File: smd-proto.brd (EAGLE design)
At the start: 79.2 x 43.9 mm, 65 parts

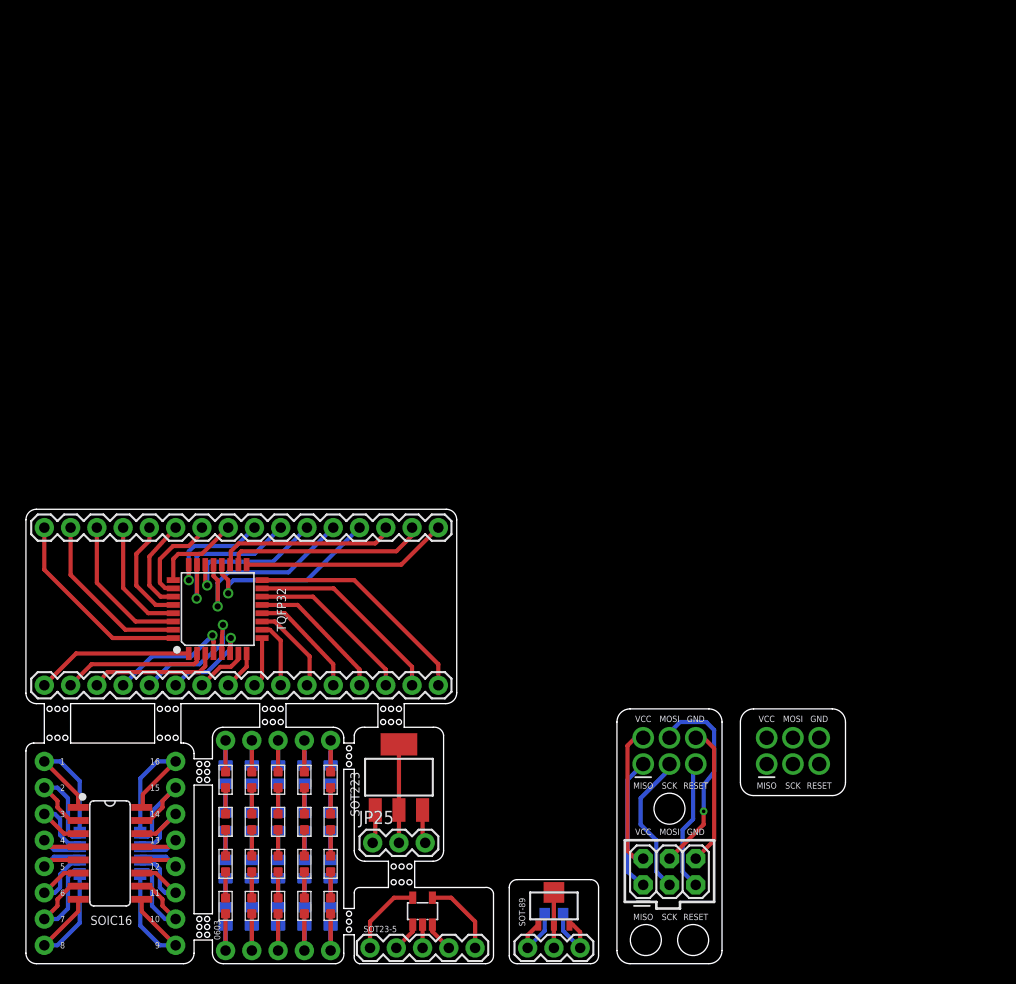
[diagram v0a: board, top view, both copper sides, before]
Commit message: Added bunch of boards and outline
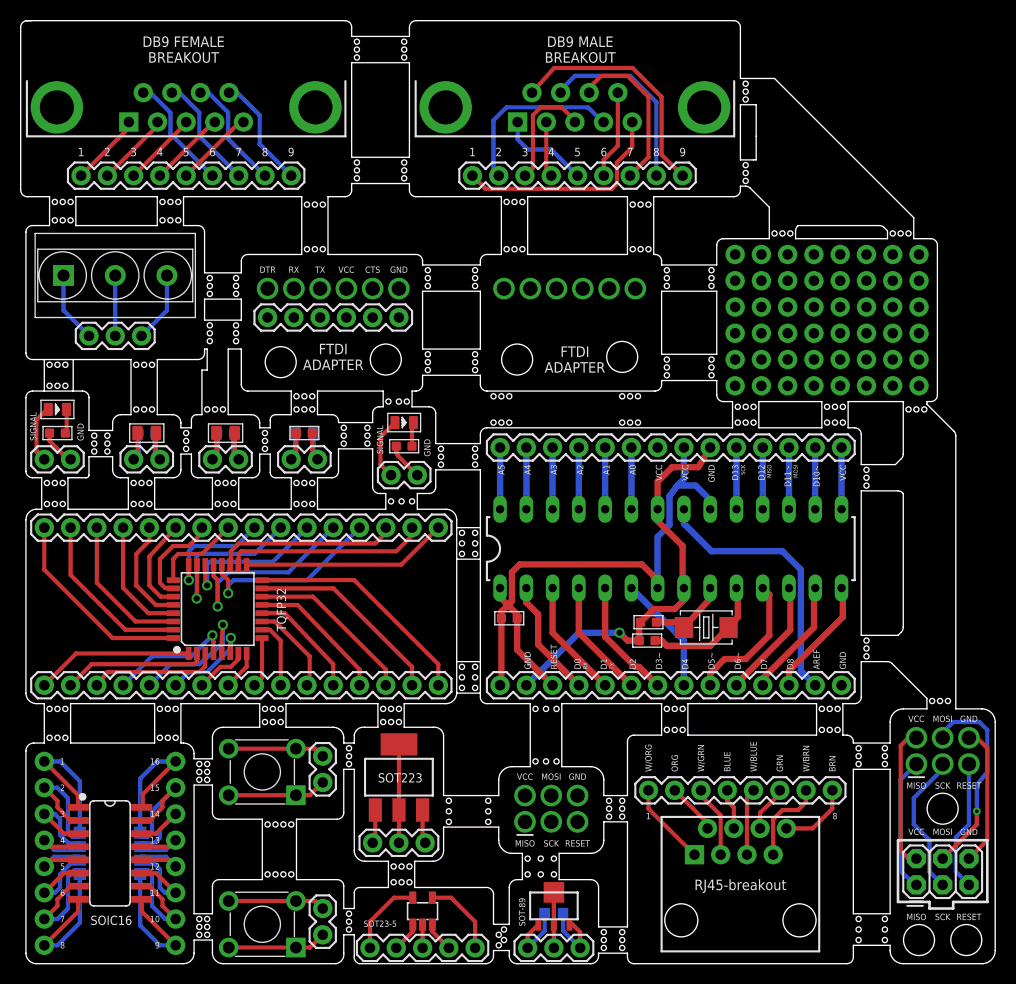
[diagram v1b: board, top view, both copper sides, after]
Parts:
- removed C10, C11, C12, C13, C14, C15, C16, C17, C18, C19, C20, C21, C3, C4, C5, C6, C7, C8, C9: 0.5PF 50V, Seeed-OPL-Capacitor:C0603
- removed C22, C23, C24, C25, C26, C27, C28, C29, C30, C31, C32, C33, C34, C35, C36, C37, C38, C39, C40: 2.2uf, Seeed-OPL-Capacitor:C0805
- added C41, C43, C45: 0.5PF 50V, Seeed-OPL-Capacitor:C0603
- added C42, C44, C46: 2.2uf, Seeed-OPL-Capacitor:C0805
- added D1, D2: RED-0805, Seeed-OPL-Diode:LED-0805
- added J1: GREEN-3P-5.0, Seeed-OPL-Connector:H3-5.0-15.5X8.0MM
- added JP15, JP17, JP19, JP20, JP27: (no value), SparkFun-Connectors:1X02
- added JP16: (no value), SparkFun-Connectors:1X09
- added JP18: FTDI_BASICPTH, SparkFun-Connectors:FTDI_BASIC
- added JP22, JP23, JP24, JP26, JP30, JP31: (no value), SparkFun-Connectors:1X08_NO_SILK
- added K1, K2: TS-1109-7, Seeed-OPL-Switch:SW4-6.2X6.2X5.0MM
- added R1, R3: 1.1M 1/10W, Seeed-OPL-Resistor:R0603
- added R2: 1K, Seeed-OPL-Resistor:R0603
- added U1: ATMEGA328P_PDIP, SparkFun-DigitalIC:DIL28-3
- added Y1: 16MHZ, Seeed-OPL-crystal-osctllator:X2-SMD-5.0X3.2X1.3MM
- C1: value 0.5PF 50V -> 22pf
- C2: value 2.2uf -> 22pf; device Seeed-OPL-Capacitor:C0805 -> Seeed-OPL-Capacitor:C0603
- JP10, JP9: device SparkFun-Connectors:1X01NS-KIT -> SparkFun-Connectors:1X14
- JP11: device SparkFun-Connectors:1X01NS-KIT -> SparkFun-Connectors:DB9_MALE
- JP12: device SparkFun-Connectors:1X01NS-KIT -> SparkFun-Connectors:1X09
- JP13: device SparkFun-Connectors:1X01NS-KIT -> SparkFun-Connectors:DB9
- JP4, JP6: device SparkFun-Connectors:1X01NS-KIT -> SparkFun-Connectors:1X02
- JP5: device SparkFun-Connectors:1X01NS-KIT -> SparkFun-Connectors:1X03
- JP7: value (none) -> RJ45; device SparkFun-Connectors:1X01NS-KIT -> SparkFun-Connectors:RJ45-8
- JP8: device SparkFun-Connectors:1X01NS-KIT -> SparkFun-Connectors:1X08_ROUND
- moved JP11 85.6 mm to (53.3, 83.8)
- moved JP13 82.7 mm to (15.7, 83.8)
- moved JP5 60.9 mm to (6.35, 61.7)
- moved JP12 56.3 mm to (43.4, 77.2)
- moved JP8 53.8 mm to (78.2, 17.8), turned to 180 degrees
- moved JP9 53.2 mm to (46.1, 50.9)
- moved JP7 47.3 mm to (69.3, 5.21)
- moved C1 43.6 mm to (60.5, 34.0), turned to 90 degrees
- moved C2 42.8 mm to (60.3, 32.3), flipped to the top, turned to 90 degrees
- moved JP6 33.8 mm to (2.03, 49.8)
- moved JP14 26.4 mm to (86.4, 8.64)
- moved JP10 19.7 mm to (46.1, 27.9)
- moved JP4 9.52 mm to (29.0, 21.1), turned to 270 degrees
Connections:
- removed net N$100: C35.2, C36.1
- removed net N$102: C18.1, C37.1, JP12.1
- removed net N$96: C13.2, C36.2, JP11.1
- removed net N$98: C33.2, C34.1
- removed net N$99: C34.2, C35.1
- new net A_A0: JP9.6, U1.23
- new net A_A1: JP9.5, U1.24
- new net A_A2: JP9.4, U1.25
- new net A_A3: JP9.3, U1.26
- new net A_A4/SDC: JP9.2, U1.27
- new net A_A5/SCL: JP9.1, U1.28
- new net A_AREF: JP10.13, U1.21
- new net A_D0/RX: JP10.4, U1.2
- new net A_D1/TX: JP10.5, U1.3
- new net A_D10~: JP9.13, U1.16
- new net A_D11~/MOSI: JP9.12, U1.17
- new net A_D2: JP10.6, U1.4
- new net A_D3~: JP10.7, U1.5
- new net A_D4: JP10.8, U1.6
- new net A_D5~: JP10.9, U1.11
- new net A_D6~: JP10.10, U1.12
- new net A_D7: JP10.11, U1.13
- new net A_D8: JP10.12, U1.14
- new net A_D9~: JP10.14, JP9.14, U1.15
- new net A_GND: C1.1, C2.1, JP10.2, JP9.9, U1.22, U1.8
- new net A_RESET: JP10.3, R2.2, U1.1
- new net A_VCC: JP10.1, JP9.8, R2.1, U1.20, U1.7
- new net D12/MISO: JP9.11, U1.18
- new net D13/SCK: JP9.10, U1.19
- new net FTDI_CTS: JP18.CTS
- new net FTDI_DTR: JP18.DTR
- new net FTDI_GND: JP18.GND
- new net FTDI_RX: JP18.RXI
- new net FTDI_TX: JP18.TXO
- new net FTDI_VCC: JP18.VCC
- new net N$108: JP27.2, R3.2
- new net N$43: C41.1, C42.1, JP15.1
- new net N$44: C41.2, C42.2, JP15.2
- new net N$45: C43.1, C44.1, JP17.1
- new net N$46: C43.2, C44.2, JP17.2
- new net N$47: C45.1, C46.1, JP19.1
- new net N$50: C45.2, C46.2, JP19.2
- new net N$52: JP4.2, K1.1, K1.4
- new net N$55: D1.+, JP6.1
- new net N$56: D1.-, R1.1
- new net N$76: JP11.1, JP12.1
- new net N$92: JP13.6, JP16.6
- net N$103: now also JP20.1, K2.2, K2.3; no longer C37.2, C38.1
- net N$104: now also JP20.2, K2.1, K2.4; no longer C38.2, C39.1
- net N$105: now also D2.+, JP27.1; no longer C39.2, C40.1
- net N$106: now also D2.-, R3.1; no longer C21.2, C40.2, JP13.1
- net N$41: now also JP4.1, K1.2, K1.3; no longer C3.2, C4.1
- net N$58: now also JP6.2, R1.2; no longer C4.2, C5.1
- net N$60: now also J1.2, JP5.2; no longer C1.2, C3.1
- net N$61: now also J1.1, JP5.1; no longer C10.1, C33.1, JP10.1
- net N$62: now also J1.3, JP5.3; no longer C6.2, C7.1
- net N$63: now also JP7.1, JP8.8; no longer C7.2, C8.1
- net N$64: now also JP7.2, JP8.7; no longer C8.2, C9.1
- net N$65: now also JP7.3, JP8.6; no longer C14.1, C29.1, JP8.1
- net N$66: now also JP7.4, JP8.5; no longer C17.2, C32.2, JP9.1
- net N$67: now also JP7.5, JP8.4; no longer C10.2, C11.1
- net N$68: now also JP7.6, JP8.3; no longer C11.2, C12.1
- net N$69: now also JP7.7, JP8.2; no longer C12.2, C13.1
- net N$72: now also JP7.8, JP8.1; no longer C14.2, C15.1
- net N$73: now also C1.2, U1.9, Y1.2; no longer C15.2, C16.1
- net N$74: now also C2.2, U1.10, Y1.1; no longer C16.2, C17.1
- net N$77: now also JP11.2, JP12.2; no longer C18.2, C19.1
- net N$78: now also JP11.3, JP12.3; no longer C19.2, C20.1
- net N$79: now also JP11.4, JP12.4; no longer C20.2, C21.1
- net N$82: now also JP11.5, JP12.5; no longer C1.1, C2.1, JP4.1
- net N$83: now also JP11.6, JP12.6; no longer C2.2, C22.1
- net N$84: now also JP11.7, JP12.7; no longer C22.2, C23.1
- net N$85: now also JP11.8, JP12.8; no longer C23.2, C24.1
- net N$86: now also JP11.9, JP12.9; no longer C24.2, C5.2, JP5.1
- net N$87: now also JP13.1, JP16.1; no longer C25.1, C6.1, JP6.1
- net N$88: now also JP13.2, JP16.2; no longer C25.2, C26.1
- net N$89: now also JP13.3, JP16.3; no longer C26.2, C27.1
- net N$90: now also JP13.4, JP16.4; no longer C27.2, C28.1
- net N$91: now also JP13.5, JP16.5; no longer C28.2, C9.2, JP7.1
- net N$93: now also JP13.7, JP16.7; no longer C29.2, C30.1
- net N$94: now also JP13.8, JP16.8; no longer C30.2, C31.1
- net N$95: now also JP13.9, JP16.9; no longer C31.2, C32.1
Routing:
- net A_VCC: track 0.00 -> 46.4 mm
- net A_GND: track 0.00 -> 39.5 mm, vias 0 -> 1
- net A_AREF: track 0.00 -> 26.3 mm
- net N$76: track 0.00 -> 21.3 mm
- net N$86: track 5.97 -> 23.2 mm
- net N$85: track 2.79 -> 18.2 mm
- net N$77: track 2.54 -> 17.3 mm
- net A_D5~: track 0.00 -> 13.2 mm
- net N$84: track 2.79 -> 15.9 mm
- net A_D3~: track 0.00 -> 11.7 mm
- net A_D8: track 0.00 -> 11.6 mm
- net A_D6~: track 0.00 -> 11.6 mm
- net A_D2: track 0.00 -> 11.5 mm
- net A_D1/TX: track 0.00 -> 11.5 mm
- net A_RESET: track 0.00 -> 11.5 mm
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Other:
- board size 79.2 x 43.9 mm -> 94.2 x 91.2 mm
- board text added: "A0"
- board text added: "A1"
- board text added: "A2"
- board text added: "A3"
- board text added: "A4"
- board text added: "A5"
- board text added: "AREF"
- board text added: "BLUE"
- board text added: "BRN"
- board text added: "CTS"
- board text added: "D0"
- board text added: "D1"
- board text added: "D10~"
- board text added: "D11~"
- board text added: "D12"
- board text added: "D13"
- board text added: "D2"
- board text added: "D3~"
- board text added: "D4"
- board text added: "D5~"
- board text added: "D6~"
- board text added: "D7"
- board text added: "D8"
- board text added: "DB9 FEMALE BREAKOUT"
- board text added: "DB9 MALE BREAKOUT"
- board text added: "DTR"
- board text added: "FTDI ADAPTER"
- board text added: "GRN"
- board text added: "ORG"
- board text added: "RJ45-breakout"
- board text added: "RX"
- board text added: "SIGNAL"
- board text added: "TX"
- board text added: "W/BLUE"
- board text added: "W/BRN"
- board text added: "W/GRN"
- board text added: "W/ORG"
- board text removed: "0603"
- board text removed: "0805"
